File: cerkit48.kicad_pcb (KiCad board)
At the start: 2 copper layers, 235.7 x 83.3 mm, 103 parts, among them J1 I2C, SW10 CherryMX, SW11 CherryMX, SW12 CherryMX, SW13 CherryMX, SW14 CherryMX, SW15 CherryMX, SW16 CherryMX, SW17 CherryMX, SW18 CherryMX, SW19 CherryMX, SW2 CherryMX, SW20 CherryMX, SW21 CherryMX, SW22 CherryMX, SW23 CherryMX, SW24 CherryMX, SW25 CherryMX, SW26 CherryMX, SW27 CherryMX, SW28 CherryMX, SW29 CherryMX, SW3 CherryMX, SW30 CherryMX, SW31 CherryMX, SW32 CherryMX, SW33 CherryMX, SW34 CherryMX, SW35 CherryMX, SW36 CherryMX, SW37 CherryMX, SW38 CherryMX, SW39 CherryMX, SW4 CherryMX, SW40 CherryMX, SW41 CherryMX, SW42 CherryMX, SW43 CherryMX, SW44 CherryMX, SW45 CherryMX, SW46 CherryMX, SW47 CherryMX, SW48 CherryMX, SW49 CherryMX, SW5 CherryMX, SW6 CherryMX, SW7 CherryMX, SW8 CherryMX, SW9 CherryMX, U1 proton_c

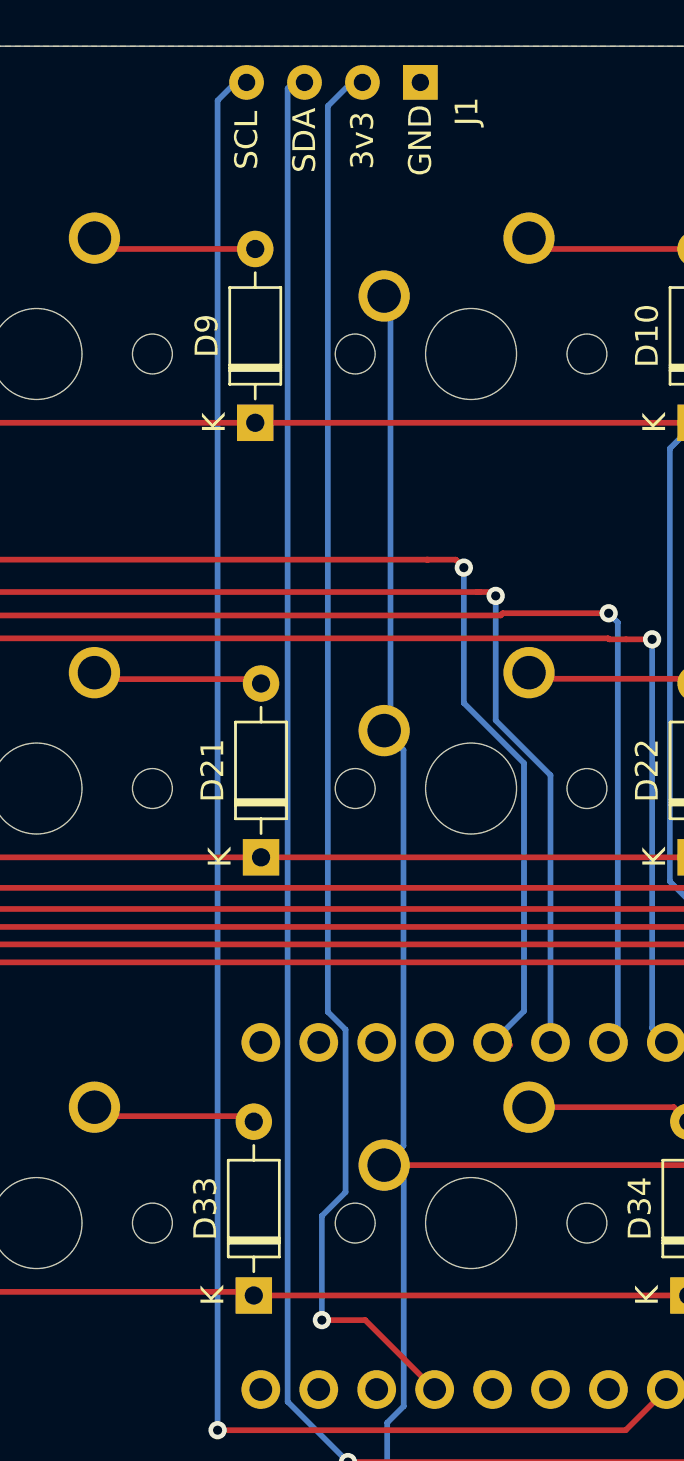
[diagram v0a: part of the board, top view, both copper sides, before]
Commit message: modified gerber files
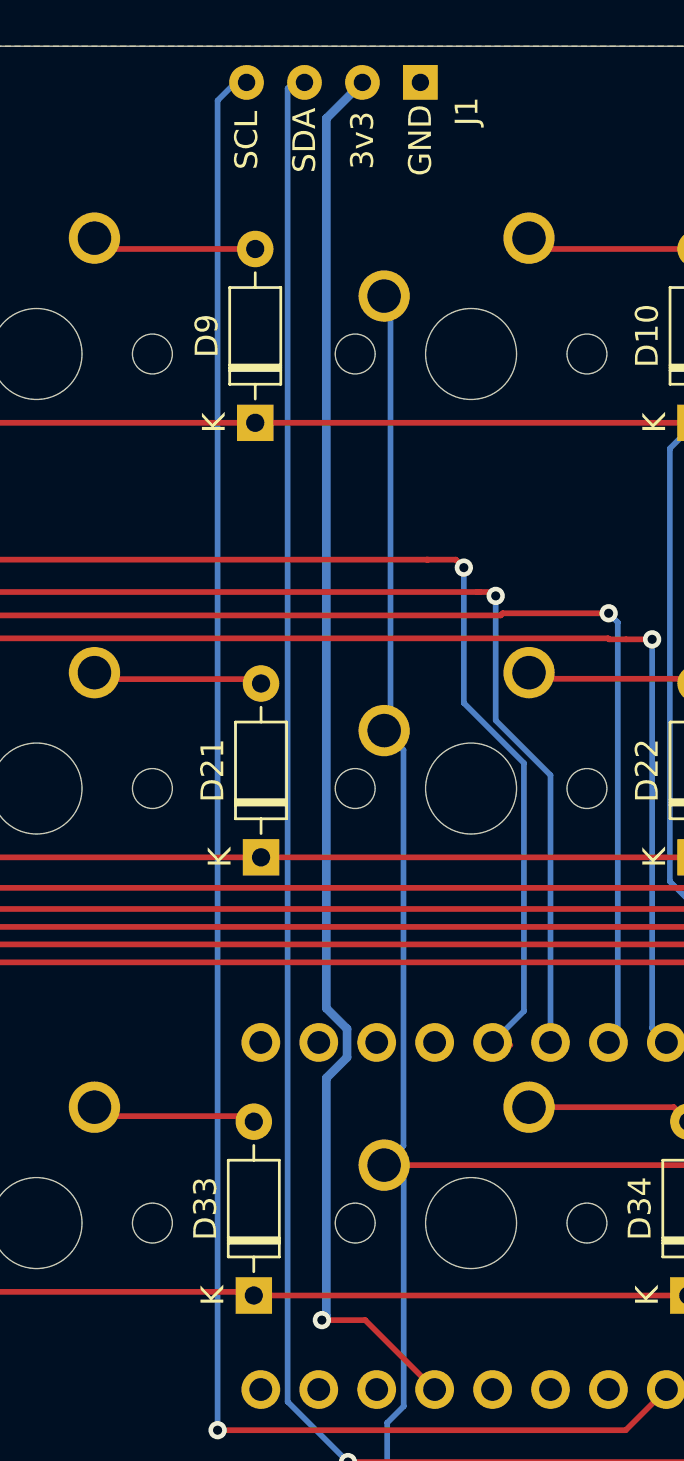
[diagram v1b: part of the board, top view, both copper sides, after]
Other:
- net class Default: trace_width 0.25 -> 0.254
- net class Power added: clearance 0.2, trace_width 0.381, via_dia 0.8, via_drill 0.4
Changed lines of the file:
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@@
     (thickness 1.6)
     (drawings 92)
-    (tracks 384)
+    (tracks 385)
     (zones 0)
     (modules 103)
@@
   (layers
     (0 F.Cu signal)
-    (31 B.Cu signal hide)
+    (31 B.Cu signal)
     (32 B.Adhes user hide)
     (33 F.Adhes user hide)
@@
   )
   (setup
-    (last_trace_width 0.25)
+    (last_trace_width 0.254)
     (trace_clearance 0.2)
     (zone_clearance 0.508)
@@
   (net_class Default "This is the default net class."
     (clearance 0.2)
-    (trace_width 0.25)
+    (trace_width 0.254)
     (via_dia 0.8)
     (via_drill 0.4)
     (uvia_dia 0.3)
     (uvia_drill 0.1)
-    (add_net 3.3V)
     (add_net COL0)
     (add_net COL1)
@@
     (add_net COL8)
     (add_net COL9)
-    (add_net GND)
     (add_net "Net-(D1-Pad2)")
     (add_net "Net-(D10-Pad2)")
@@
     (add_net SDA)
   )
+  (net_class Power ""
+    (clearance 0.2)
+    (trace_width 0.381)
+    (via_dia 0.8)
+    (via_drill 0.4)
+    (uvia_dia 0.3)
+    (uvia_drill 0.1)
+    (add_net 3.3V)
+    (add_net GND)
+  )
   (module MountingHole:MountingHole_3.2mm_M3 (layer F.Cu)
     (at 256.54 54.61 180)
@@
   (segment (start 199.920001 111.020001) (end 199.920001 53.444999) (width 0.25) (layer B.Cu) (net 54))
   (segment (start 202.565 113.665) (end 199.920001 111.020001) (width 0.25) (layer B.Cu) (net 54))
-  (segment (start 202.460001 101.833997) (end 201.422 102.871998) (width 0.25) (layer B.Cu) (net 55))
-  (segment (start 202.460001 94.705999) (end 202.460001 101.833997) (width 0.25) (layer B.Cu) (net 55))
-  (segment (start 201.682499 93.928497) (end 202.460001 94.705999) (width 0.25) (layer B.Cu) (net 55))
-  (segment (start 203.2 52.705) (end 201.682499 54.222501) (width 0.25) (layer B.Cu) (net 55))
-  (segment (start 201.682499 54.222501) (end 201.682499 93.928497) (width 0.25) (layer B.Cu) (net 55))
-  (segment (start 201.422 102.871998) (end 201.422 107.442) (width 0.25) (layer B.Cu) (net 55))
   (segment (start 201.422 107.442) (end 201.422 107.442) (width 0.25) (layer B.Cu) (net 55))
   (via (at 201.422 107.442) (size 0.8) (drill 0.4) (layers F.Cu B.Cu) (net 55))
   (segment (start 203.322 107.442) (end 206.365 110.485) (width 0.25) (layer F.Cu) (net 55))
   (segment (start 201.422 107.442) (end 203.322 107.442) (width 0.25) (layer F.Cu) (net 55))
+  (segment (start 202.525501 94.674559) (end 202.525501 95.924499) (width 0.381) (layer B.Cu) (net 55))
+  (segment (start 201.616999 93.766057) (end 202.525501 94.674559) (width 0.381) (layer B.Cu) (net 55))
+  (segment (start 203.2 53.18125) (end 201.616999 54.764251) (width 0.381) (layer B.Cu) (net 55))
+  (segment (start 201.616999 54.764251) (end 201.616999 93.766057) (width 0.381) (layer B.Cu) (net 55))
+  (segment (start 201.616999 107.247001) (end 201.422 107.442) (width 0.381) (layer B.Cu) (net 55))
+  (segment (start 201.616999 96.833001) (end 201.616999 107.247001) (width 0.381) (layer B.Cu) (net 55))
+  (segment (start 202.525501 95.924499) (end 201.616999 96.833001) (width 0.381) (layer B.Cu) (net 55))
   (segment (start 206.365 95.24) (end 206.375 95.25) (width 0.25) (layer B.Cu) (net 56))
   (segment (start 32.749463 81.75035) (end 32.870936 81.871823) (width 0.25) (layer B.Cu) (net 57))
@@
   (segment (start 242.2525 100.6475) (end 243.100001 101.495001) (width 0.25) (layer B.Cu) (net 68))
   (segment (start 231.765 95.24) (end 231.775 95.25) (width 0.25) (layer F.Cu) (net 73))
-  (zone (net 56) (net_name GND) (layer F.Cu) (hatch edge 0.508)
+  (zone (net 56) (net_name GND) (layer B.Cu) (hatch edge 0.508)
     (connect_pads (clearance 0.508))
     (min_thickness 0.254)
@@
     )
   )
-  (zone (net 56) (net_name GND) (layer B.Cu) (hatch edge 0.508)
+  (zone (net 56) (net_name GND) (layer F.Cu) (hatch edge 0.508)
     (connect_pads (clearance 0.508))
     (min_thickness 0.254)
